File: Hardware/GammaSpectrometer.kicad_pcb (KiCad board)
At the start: 4 copper layers, 100 x 100 mm, 275 parts, among them J1801 USB_B_Micro, U1002 LT3042, U1101 REF3220AMDBVREP, U1201 MX25L1606EM1I-12G, U1301 XLH736065.000000I, U1302 5PB1102PGGK, U1601 TPS7A4901, U1801 CH340X, U2001 OPA690xDBV, U2002 AD8139, U2101 OPA690xDBV, U2102 AD8139, U401 MCP4725A0T-E/CH, U402 MCP3221, U501 LT8330IS6, U601 ICE40HX4K-TQ144, U802 LT3093, U803 LT8330IS6, U901 NCP163ASN330T1G (3v3), U902 AP2112K-3.3, U903 AP2112K-1.2, U904 AP2112K-2.5, U905 TPS62932

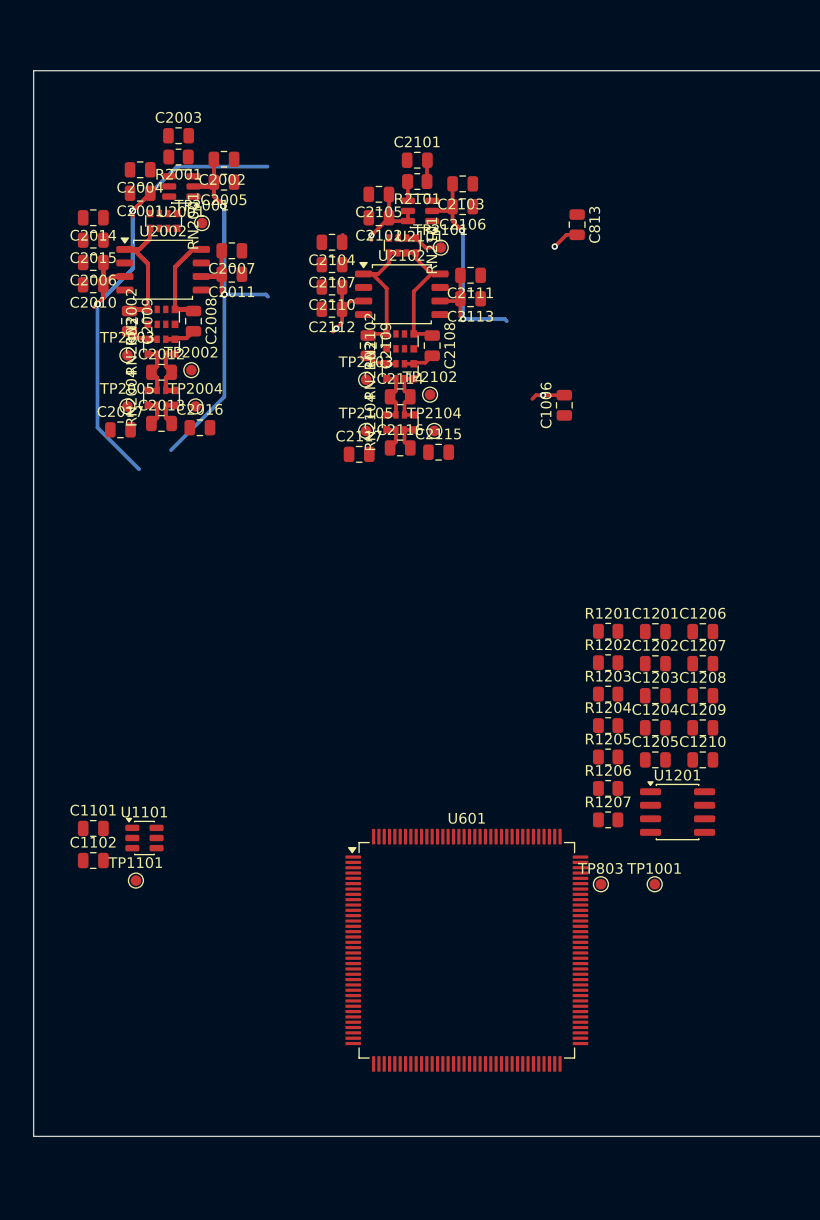
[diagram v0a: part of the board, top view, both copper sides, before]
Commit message: emi
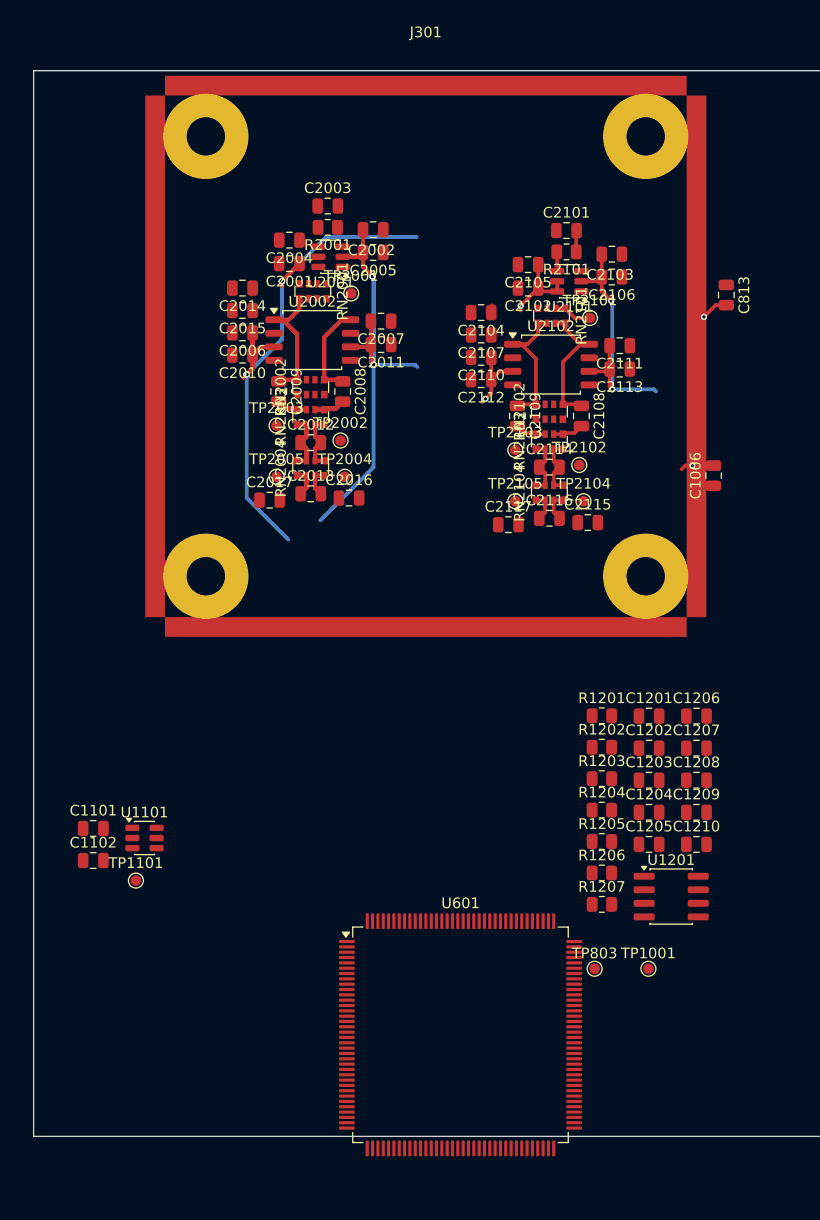
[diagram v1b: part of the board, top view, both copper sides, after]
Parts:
- added J301: RFShield_TwoPieces, GammaSpectrometer:BUD_CU-470_Shield, F.Cu at (131.8, 51.8)
- moved C2117 15.5 mm to (139.6, 67.6)
- moved C2115 15.5 mm to (147.0, 67.4)
- moved TP2104 15.5 mm to (146.6, 65.4)
- moved C1006 15.5 mm to (158.8, 63.0)
- moved C2001 15.5 mm to (119.0, 43.1)
- moved C2003 15.5 mm to (122.6, 37.7)
- moved C2004 15.5 mm to (119.0, 40.9)
- moved C2005 15.5 mm to (126.9, 42.1)
- moved C2006 15.5 mm to (114.6, 49.6)
- moved C2007 15.5 mm to (127.6, 48.5)
- moved C2008 15.5 mm to (124.0, 55.1)
- moved C2009 15.5 mm to (118.0, 55.1)
- moved C2011 15.5 mm to (127.6, 50.7)
- moved C2012 15.5 mm to (121.0, 59.9)
- moved C2013 15.5 mm to (121.0, 64.7)
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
